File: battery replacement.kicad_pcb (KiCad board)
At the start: 2 copper layers, 22.5 x 11.1 mm, 15 parts, among them U1 GP3134_C48997205

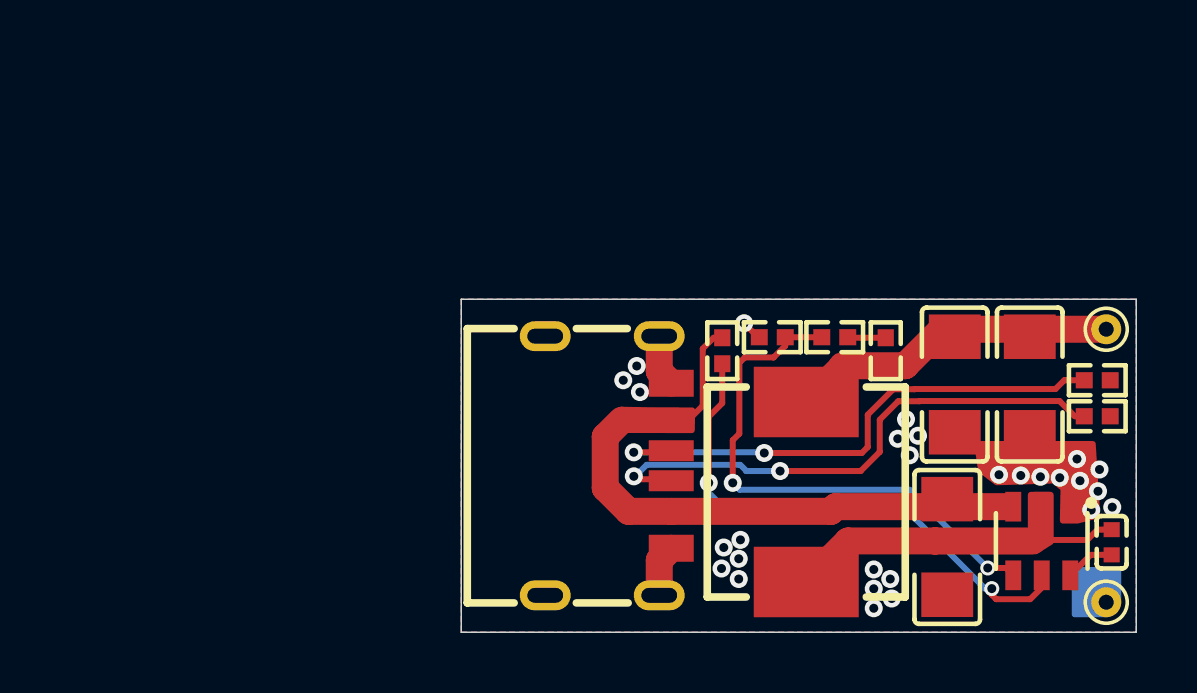
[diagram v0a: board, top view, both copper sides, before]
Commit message: prelim. 10x25mm ~ 180pcs
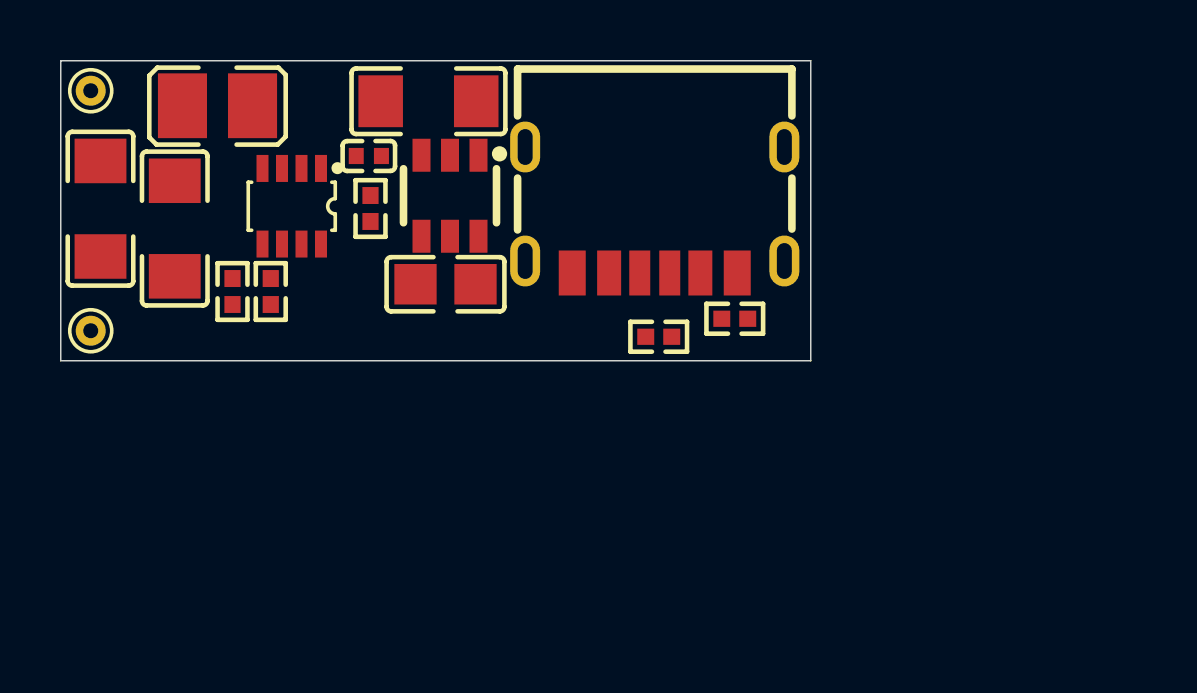
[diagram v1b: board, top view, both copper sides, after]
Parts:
- removed R4: 10k, JLCImport:0402WGF1002TCE
- added C7: 4.7uF, JLCImport:CL21A475KAQNNNE, F.Cu at (139.6, 45.5)
- added U2: Y4203-ADJM6R, JLCImport:Y4203-ADJM6R, F.Cu at (139.7, 42.5)
- L1: value 4.7uH -> 470nH; footprint JLCImport:BMQA000606304R7MA1 -> JLCImport:TMS252012ALM-R47MTAA
- R1: value 10k -> 100k; footprint JLCImport:0402WGF1002TCE -> JLCImport:0402WGF1003TCE
- R2: value 20k -> 549k; footprint JLCImport:0402WGF2002TCE -> JLCImport:0402WGF5493TCE
- R3: value 20k -> 100k; footprint JLCImport:0402WGF2002TCE -> JLCImport:0402WGF1003TCE
- U1: value GP3134_C48997205 -> RT5788BGJ8F; footprint JLCImport:GP3134_C48997205 -> JLCImport:RT5788BGJ8F
- moved TP2 35.0 mm to (127.8, 47.0)
- moved TP1 34.8 mm to (127.8, 39.0)
- moved C4 29.1 mm to (128.1, 42.9)
- moved C3 29.0 mm to (130.6, 43.6)
- moved C2 27.9 mm to (137.0, 41.2), turned to 0 degrees
- moved U1 27.4 mm to (134.4, 42.9)
- moved L1 23.5 mm to (132.0, 39.5), turned to 180 degrees
- moved C1 22.8 mm to (139.0, 39.4), turned to 180 degrees
- moved R2 21.9 mm to (132.5, 45.7), turned to 90 degrees
- moved R3 16.1 mm to (137.1, 42.9), turned to 90 degrees
- moved R1 15.2 mm to (133.8, 45.7)
- moved R5 14.9 mm to (146.7, 47.2)
- moved R6 12.3 mm to (149.2, 46.6)
- moved USB1 8.66 mm to (146.6, 43.0), turned to 180 degrees
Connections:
- C1 pad 1: +5V -> GND
- C1 pad 2: GND -> +5V
- C2 pad 1: /SW -> +5V
- C2 pad 2: /BS -> GND
- C3 pad 2: /V_OUT -> /VOUT
- C4 pad 2: /V_OUT -> /VOUT
- L1 pad 1: /SW -> /LX
- L1 pad 2: /V_OUT -> /VOUT
- R1 pad 1: /EN -> /FB
- R1 pad 2: +5V -> /AGND
- R2 pad 1: Net-(R2-Pad1) -> /FB
- R2 pad 2: /V_OUT -> /VOUT
- R3 pad 1: /FB -> /EN
- R3 pad 2: Net-(R2-Pad1) -> +5V
- TP1 pad 1: /V_OUT -> /VOUT
- U1 pad 1: GND -> unconnected-(U1-PGOOD-Pad1)
- U1 pad 2: /SW -> +5V
- U1 pad 3: +5V -> /LX
- U1 pad 4: /FB -> /PGND
- U1 pad 5: /EN -> /VOUT
- U1 pad 6: /BS -> /AGND
- USB1 pad A9: +5V -> /VBUS
- USB1 pad B9: +5V -> /VBUS
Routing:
- net +5V: track 20.2 -> 0.00 mm
- net Net-(USB1-CC1): track 18.4 -> 0.00 mm, vias 2 -> 0
- net /FB: track 18.0 -> 0.00 mm, vias 2 -> 0
- net Net-(USB1-CC2): track 17.9 -> 0.00 mm, vias 2 -> 0
- net /EN: track 17.7 -> 0.00 mm, vias 2 -> 0
- net /V_OUT: track 11.0 -> 0.00 mm
- net /SW: track 10.6 -> 0.00 mm
- net GND: track 4.17 -> 0.00 mm, vias 28 -> 0
- net /BS: track 1.66 -> 0.00 mm
- net Net-(R2-Pad1): track 1.27 -> 0.00 mm
- removed copper zone on B.Cu, net GND
- removed copper zone on F.Cu, net GND
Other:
- board size 22.5 x 11.1 mm -> 25 x 10 mm
